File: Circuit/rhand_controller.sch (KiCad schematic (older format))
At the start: 16 parts, among them P1 RU_ADC, P2 LU_ADC, P3 RV_ADC, P4 LV_ADC, P5 RW_ADC, P6 LW_ADC, P7 BLUETOOTH, U1 STM32F042, U2 IM315TX

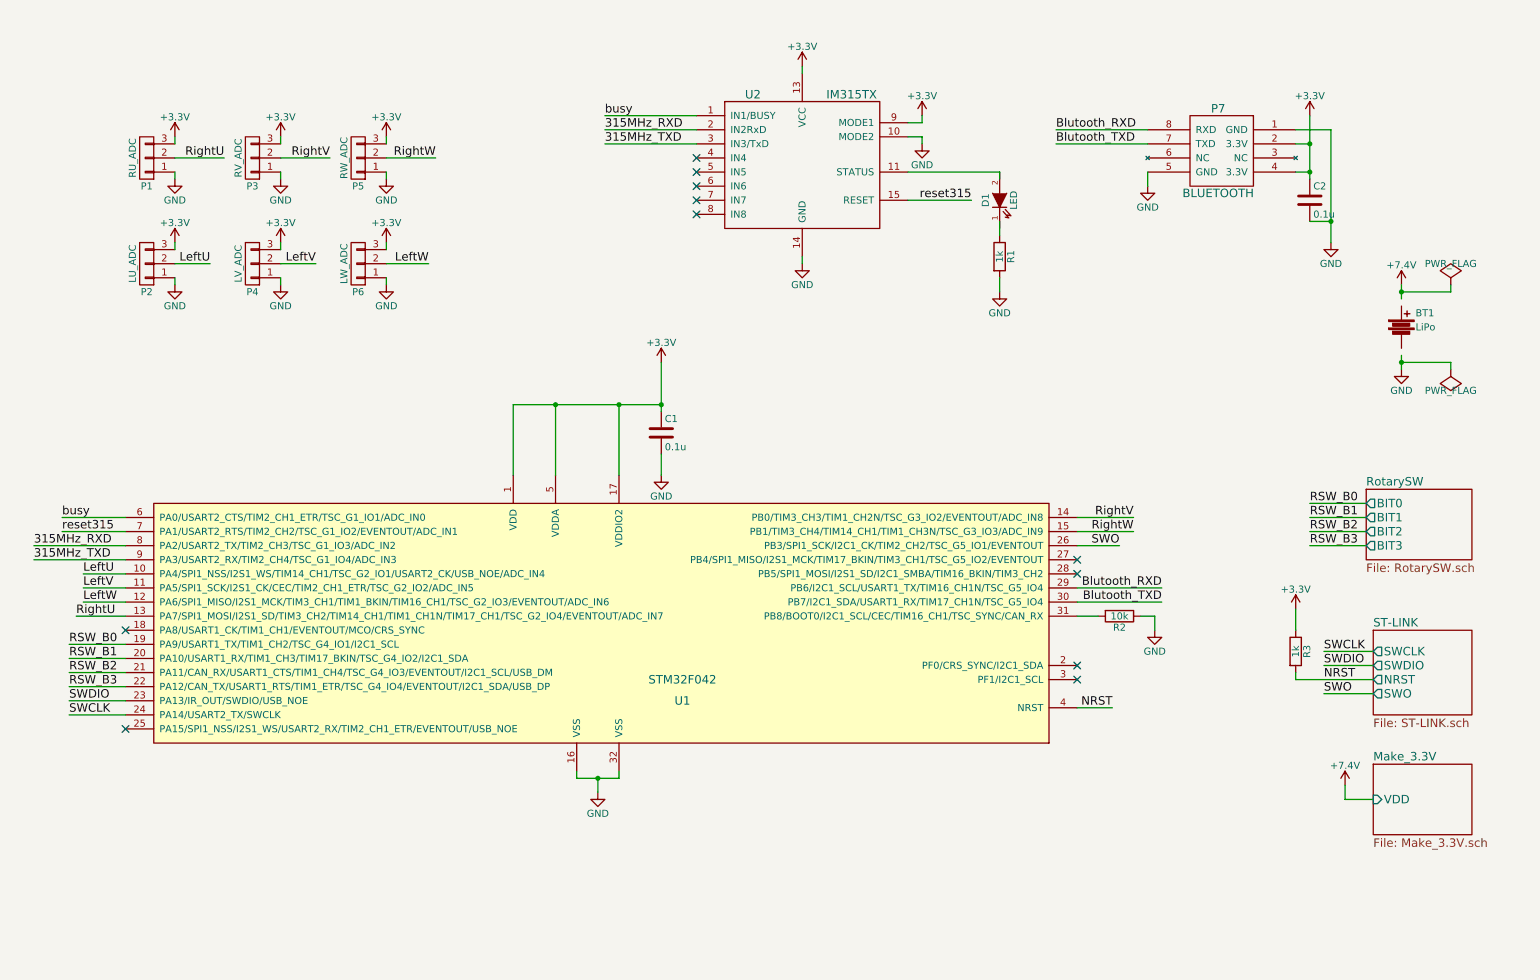
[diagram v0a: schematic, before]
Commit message: 機能の追加
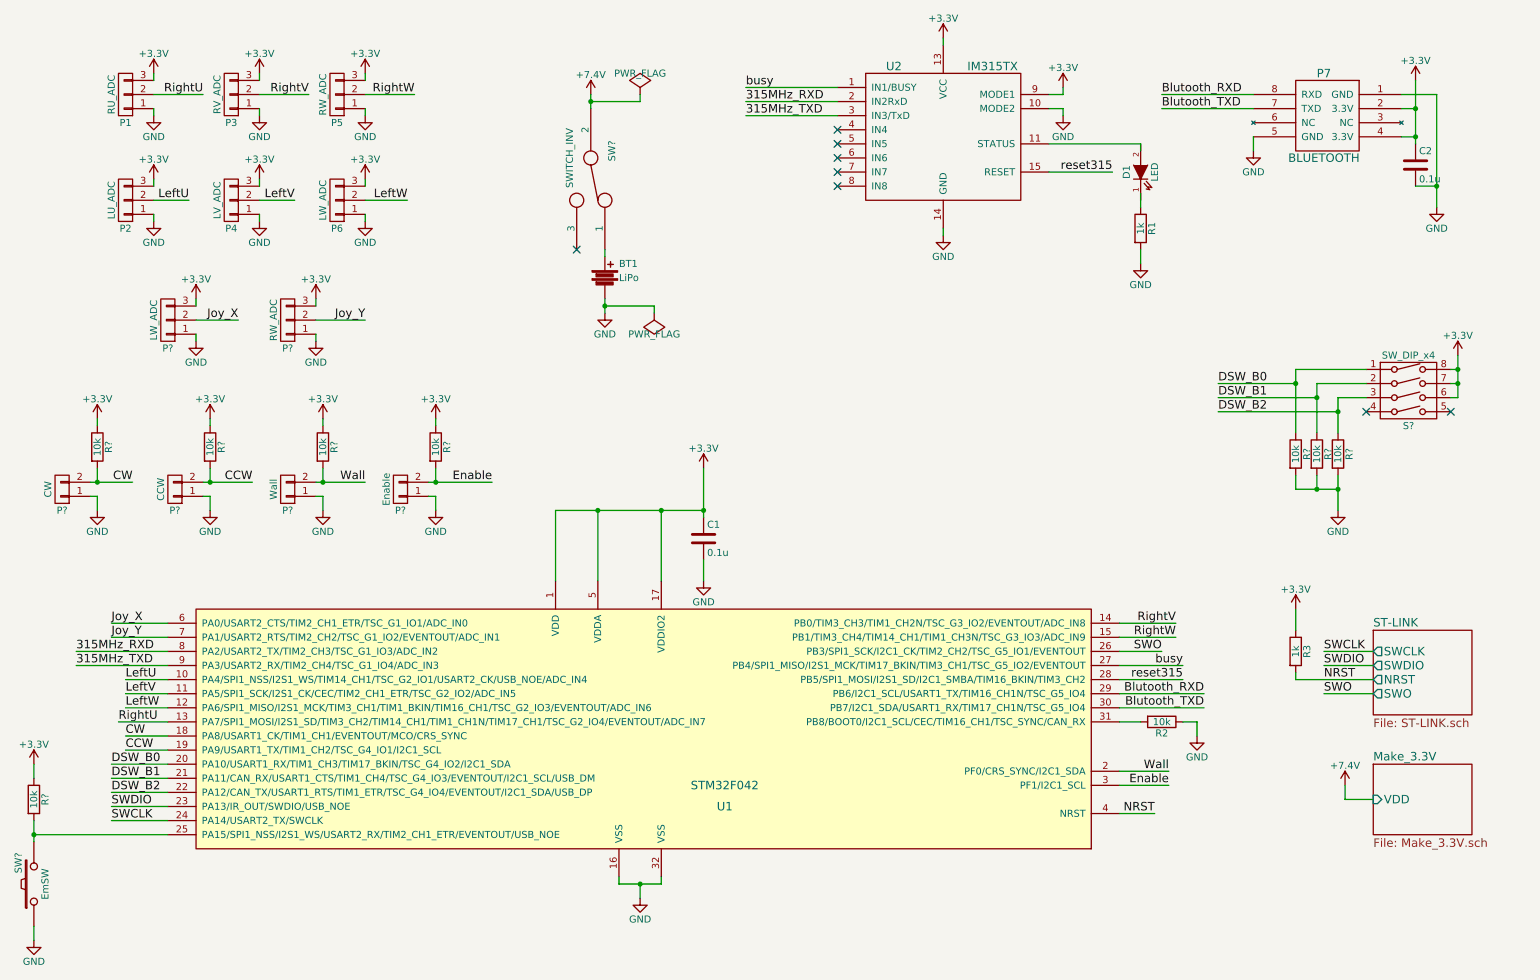
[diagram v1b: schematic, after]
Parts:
- added P?: RW_ADC, symbol CONN_01X03
- added P?: LW_ADC, symbol CONN_01X03
- added P?: CW, symbol CONN_01X02
- added P?: CCW, symbol CONN_01X02
- added P?: Wall, symbol CONN_01X02
- added P?: Enable, symbol CONN_01X02
- added R? (x8): 10k, symbol R
- added S?: SW_DIP_x4, symbol SW_DIP_x4
- added SW?: EmSW, symbol SW_PUSH
- added SW?: SWITCH_INV, symbol SWITCH_INV
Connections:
- net labels added: CCW, CW, DSW_B0, DSW_B1, DSW_B2, Enable, Joy_X, Joy_Y, Wall
- net labels removed: RSW_B0, RSW_B1, RSW_B2, RSW_B3
- wire segments 92 -> 141
- no-connect marks 11 -> 8
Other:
- moved on the sheet: BT1, C1, C2, D1, P1, P2, P3, P4, P5, P6, P7, R1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
